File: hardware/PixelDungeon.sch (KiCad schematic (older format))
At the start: 51 parts

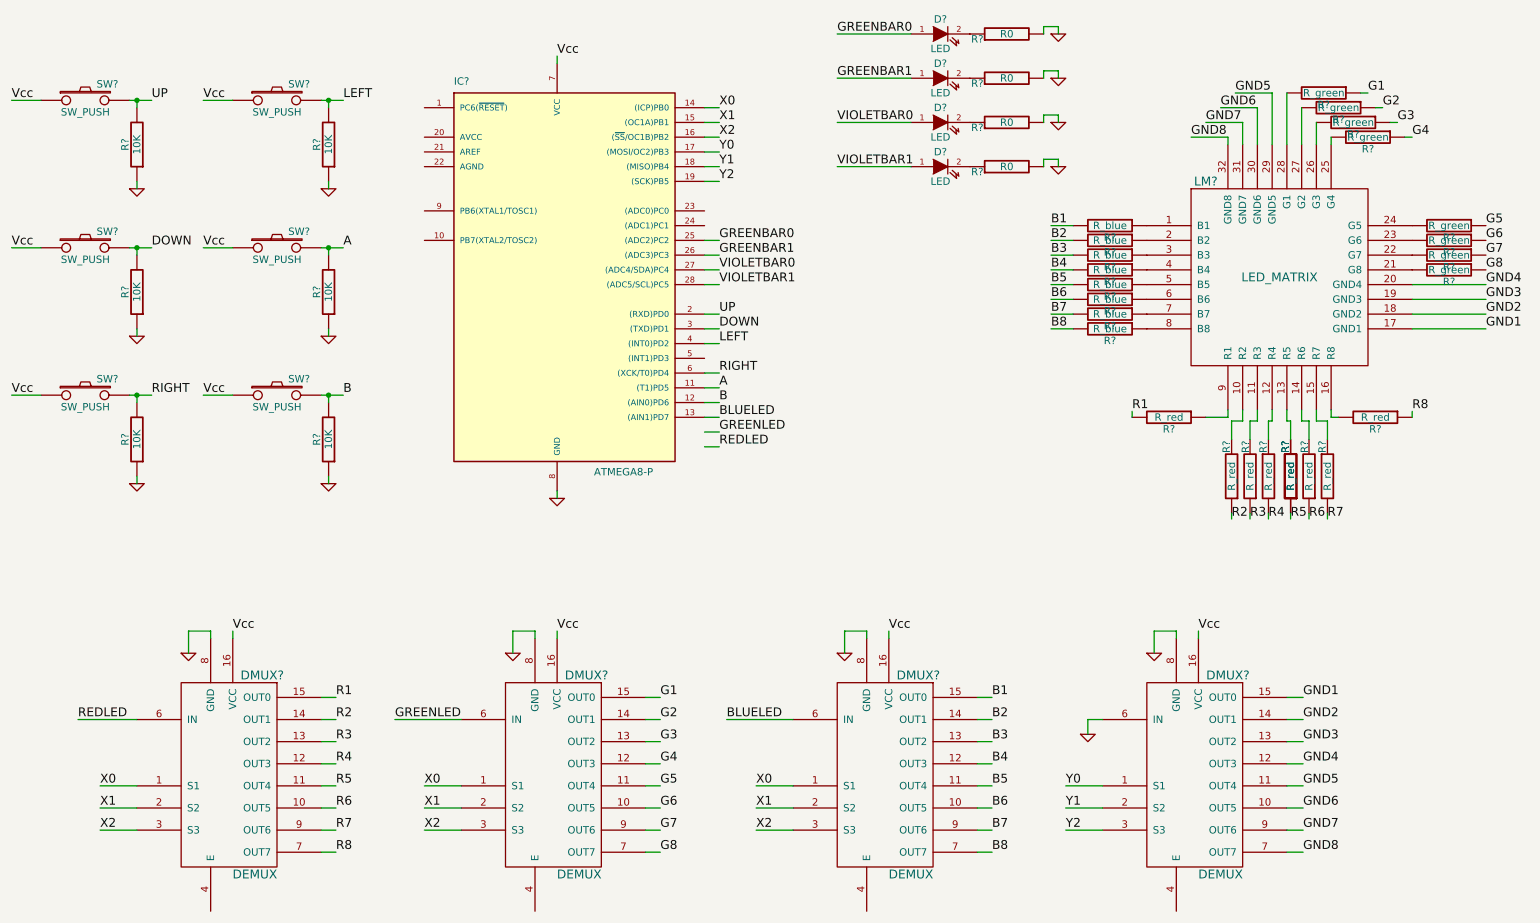
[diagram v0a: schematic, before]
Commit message: Working on schematics and PCB
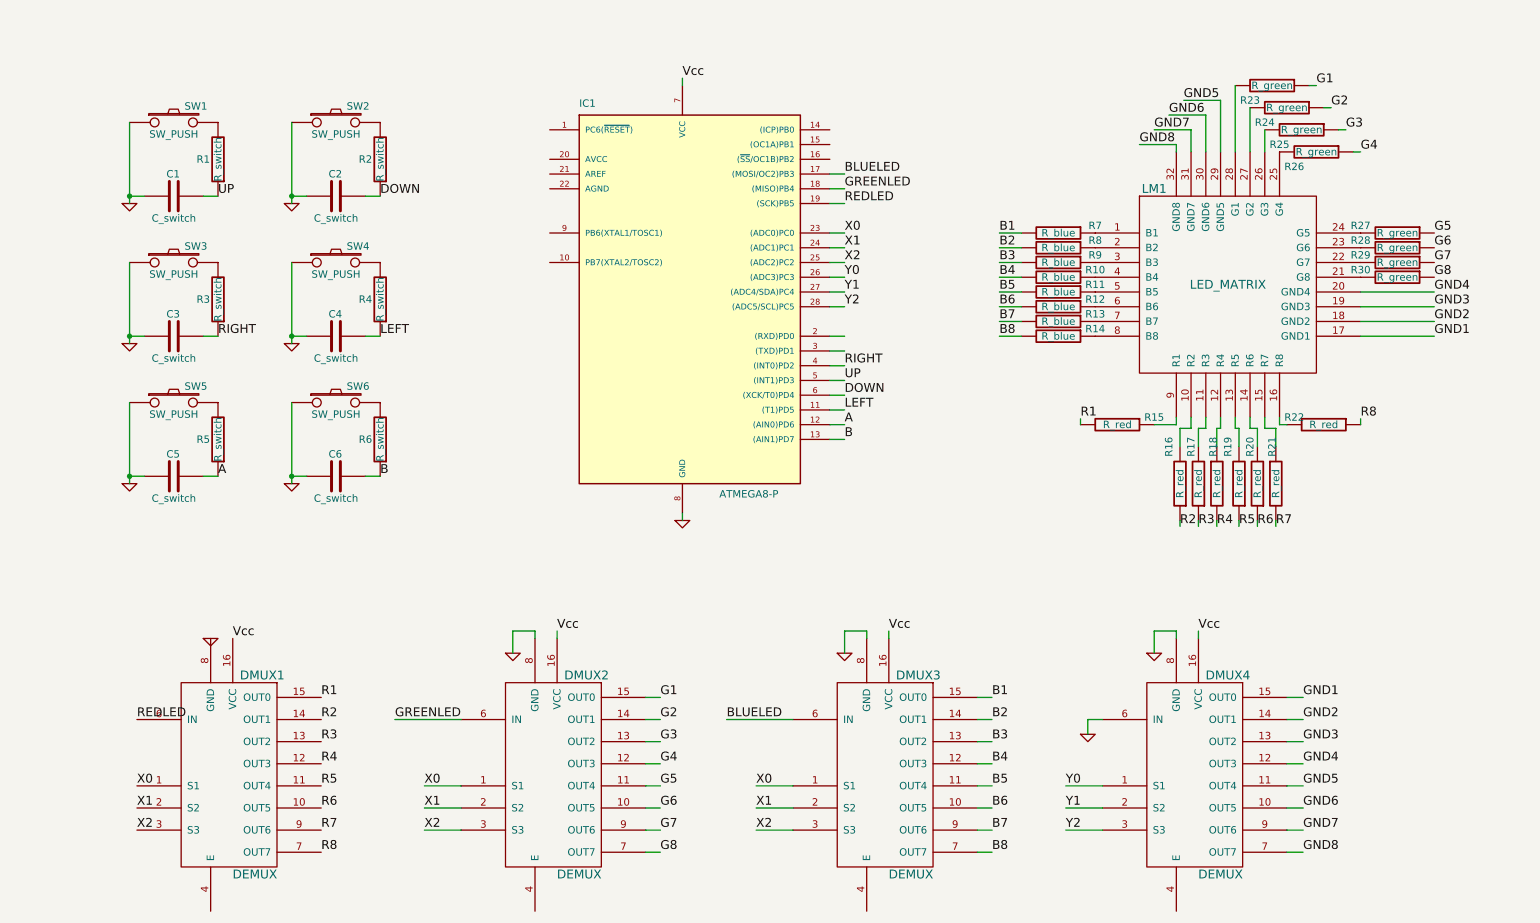
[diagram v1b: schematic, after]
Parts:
- removed D? (x4): LED, symbol LED
- removed R? (x6): 10K, symbol R
- removed R?: R_red, symbol R
- removed R? (x4): R0, symbol R
- removed SW? (x6): SW_PUSH, symbol SW_PUSH
- added C1, C2, C3, C4, C5, C6: C_switch, symbol C
- added R1, R2, R3, R4, R5, R6: R_switch, symbol R
- added SW1, SW2, SW3, SW4, SW5, SW6: SW_PUSH, symbol SW_PUSH
- gave numbers to parts that had none: 30
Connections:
- net GREENBAR0 is gone; now on net X2: IC1.25 ((ADC2)PC2)
- net GREENBAR1 is gone; now on net Y0: IC1.26 ((ADC3)PC3)
- net VIOLETBAR0 is gone; now on net Y1: IC1.27 ((ADC4/SDA)PC4)
- net VIOLETBAR1 is gone; now on net Y2: IC1.28 ((ADC5/SCL)PC5)
- net A: now also IC1.12 ((AIN0)PD6), C5.1, R5.1; no longer IC1.11 ((T1)PD5)
- net B: now also IC1.13 ((AIN1)PD7), C6.1, R6.1; no longer IC1.12 ((AIN0)PD6)
- net BLUELED: now also IC1.17 ((MOSI/OC2)PB3); no longer IC1.13 ((AIN1)PD7)
- net DOWN: now also IC1.6 ((XCK/T0)PD4), C2.1, R2.1; no longer IC1.3 ((TXD)PD1)
- net GND: now also C1.2, C2.2, C3.2, C4.2, C5.2, C6.2, SW1.1, SW2.1, SW3.1, SW4.1, SW5.1, SW6.1
- net GREENLED: now also IC1.18 ((MISO)PB4)
- net LEFT: now also IC1.11 ((T1)PD5), C4.1, R4.1; no longer IC1.4 ((INT0)PD2)
- net REDLED: now also IC1.19 ((SCK)PB5)
- net RIGHT: now also IC1.4 ((INT0)PD2), C3.1, R3.1; no longer IC1.6 ((XCK/T0)PD4)
- net UP: now also IC1.5 ((INT1)PD3), C1.1, R1.1; no longer IC1.2 ((RXD)PD0)
- net X0: now also IC1.23 ((ADC0)PC0); no longer IC1.14 ((ICP)PB0)
- net X1: now also IC1.24 ((ADC1)PC1); no longer IC1.15 ((OC1A)PB1)
- net X2: no longer IC1.16 ((~SS~/OC1B)PB2)
- net Y0: no longer IC1.17 ((MOSI/OC2)PB3)
- net Y1: no longer IC1.18 ((MISO)PB4)
- net Y2: no longer IC1.19 ((SCK)PB5)
- new net: R1.2, SW1.2
- new net: R2.2, SW2.2
- new net: R6.2, SW6.2
- new net: R5.2, SW5.2
- new net: R3.2, SW3.2
- new net: R4.2, SW4.2
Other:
- moved on the sheet: IC1, LM1, R10, R11, R12, R13, R14, R15, R16, R17, R18, R19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

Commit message: More work on schematics and PCB, need to think a bit more about doing a cleaner wiring cause it's a mess...
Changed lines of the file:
@@
-EESchema Schematic File Version 2  date Sat Mar 22 19:42:48 2014
+EESchema Schematic File Version 2  date dim. 23 mars 2014 22:53:43 CET
 LIBS:power
 LIBS:device
@@
 UP
 Wire Wire Line
-	2750 3100 2750 3050
-Wire Wire Line
-	2750 3050 2750 2550
+	2750 3100 2750 2550
 Wire Wire Line
 	2850 3050 2750 3050
@@
 	1750 3050 1650 3050
 Wire Wire Line
-	1650 3100 1650 3050
-Wire Wire Line
-	1650 3050 1650 2550
-Wire Wire Line
-	1650 4050 1650 4000
-Wire Wire Line
-	1650 4000 1650 3500
+	1650 3100 1650 2550
+Wire Wire Line
+	1650 4050 1650 3500
 Wire Wire Line
 	1750 4000 1650 4000
@@
 	2850 4000 2750 4000
 Wire Wire Line
-	2750 4050 2750 4000
-Wire Wire Line
-	2750 4000 2750 3500
-Wire Wire Line
-	2750 2150 2750 2100
-Wire Wire Line
-	2750 2100 2750 1600
+	2750 4050 2750 3500
+Wire Wire Line
+	2750 2150 2750 1600
 Wire Wire Line
 	2850 2100 2750 2100
@@
 	1750 2100 1650 2100
 Wire Wire Line
-	1650 2150 1650 2100
-Wire Wire Line
-	1650 2100 1650 1600
+	1650 2150 1650 1600
 Wire Wire Line
 	6500 1950 6400 1950
@@
 LEFT
 $Comp
-L GND #PWR6
+L GND #PWR01
 U 1 1 532DBD18
 P 2750 3100
-F 0 "#PWR6" H 2750 3100 30  0001 C CNN
+F 0 "#PWR01" H 2750 3100 30  0001 C CNN
 F 1 "GND" H 2750 3030 30  0001 C CNN
 	1    2750 3100
@@
 $EndComp
 $Comp
-L GND #PWR2
+L GND #PWR02
 U 1 1 532DBD13
 P 1650 3100
-F 0 "#PWR2" H 1650 3100 30  0001 C CNN
+F 0 "#PWR02" H 1650 3100 30  0001 C CNN
 F 1 "GND" H 1650 3030 30  0001 C CNN
 	1    1650 3100
@@
 A
 $Comp
-L GND #PWR3
+L GND #PWR03
 U 1 1 532DBCE7
 P 1650 4050
-F 0 "#PWR3" H 1650 4050 30  0001 C CNN
+F 0 "#PWR03" H 1650 4050 30  0001 C CNN
 F 1 "GND" H 1650 3980 30  0001 C CNN
 	1    1650 4050
@@
 $EndComp
 $Comp
-L GND #PWR7
+L GND #PWR04
 U 1 1 532DBCE2
 P 2750 4050
-F 0 "#PWR7" H 2750 4050 30  0001 C CNN
+F 0 "#PWR04" H 2750 4050 30  0001 C CNN
 F 1 "GND" H 2750 3980 30  0001 C CNN
 	1    2750 4050
@@
 DOWN
 $Comp
-L GND #PWR5
+L GND #PWR05
 U 1 1 532DBCC1
 P 2750 2150
-F 0 "#PWR5" H 2750 2150 30  0001 C CNN
+F 0 "#PWR05" H 2750 2150 30  0001 C CNN
 F 1 "GND" H 2750 2080 30  0001 C CNN
 	1    2750 2150
@@
 $EndComp
 $Comp
-L GND #PWR1
+L GND #PWR06
 U 1 1 532DBA23
 P 1650 2150
-F 0 "#PWR1" H 1650 2150 30  0001 C CNN
+F 0 "#PWR06" H 1650 2150 30  0001 C CNN
 F 1 "GND" H 1650 2080 30  0001 C CNN
 	1    1650 2150
@@
 X0
 $Comp
-L GND #PWR9
+L GND #PWR07
 U 1 1 50195127
 P 5400 4300
-F 0 "#PWR9" H 5400 4300 30  0001 C CNN
+F 0 "#PWR07" H 5400 4300 30  0001 C CNN
 F 1 "GND" H 5400 4230 30  0001 C CNN
 	1    5400 4300
@@
 Vcc
 $Comp
-L GND #PWR11
+L GND #PWR08
 U 1 1 4E2A8C9C
 P 8150 5750
-F 0 "#PWR11" H 8150 5750 30  0001 C CNN
+F 0 "#PWR08" H 8150 5750 30  0001 C CNN
 F 1 "GND" H 8150 5680 30  0001 C CNN
 	1    8150 5750
@@
 R1
 $Comp
-L GND #PWR12
+L GND #PWR09
 U 1 1 4E233023
 P 8600 5200
-F 0 "#PWR12" H 8600 5200 30  0001 C CNN
+F 0 "#PWR09" H 8600 5200 30  0001 C CNN
 F 1 "GND" H 8600 5130 30  0001 C CNN
 	1    8600 5200
@@
 $EndComp
 $Comp
-L GND #PWR10
+L GND #PWR010
 U 1 1 4E23301F
 P 6500 5200
-F 0 "#PWR10" H 6500 5200 30  0001 C CNN
+F 0 "#PWR010" H 6500 5200 30  0001 C CNN
 F 1 "GND" H 6500 5130 30  0001 C CNN
 	1    6500 5200
@@
 $EndComp
 $Comp
-L GND #PWR8
+L GND #PWR011
 U 1 1 4E233019
 P 4250 5200
-F 0 "#PWR8" H 4250 5200 30  0001 C CNN
+F 0 "#PWR011" H 4250 5200 30  0001 C CNN
 F 1 "GND" H 4250 5130 30  0001 C CNN
 	1    4250 5200
@@
 $EndComp
 $Comp
-L GND #PWR4
+L GND #PWR012
 U 1 1 4E233016
 P 2200 5100
-F 0 "#PWR4" H 2200 5100 30  0001 C CNN
+F 0 "#PWR012" H 2200 5100 30  0001 C CNN
 F 1 "GND" H 2200 5030 30  0001 C CNN
 	1    2200 5100
